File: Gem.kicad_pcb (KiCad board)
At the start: 2 copper layers, 56 x 54 mm, 40 parts, among them IC1 AD8226, IC2 AD8538, M1 ALLSENSORS-A6AAF-CUTLEADS, M2 DIAVOLINO, M6 ADAFRUIT-GPS-MOD, U1 ADS1115, U2 TCR2EF, U3 Micro-SD

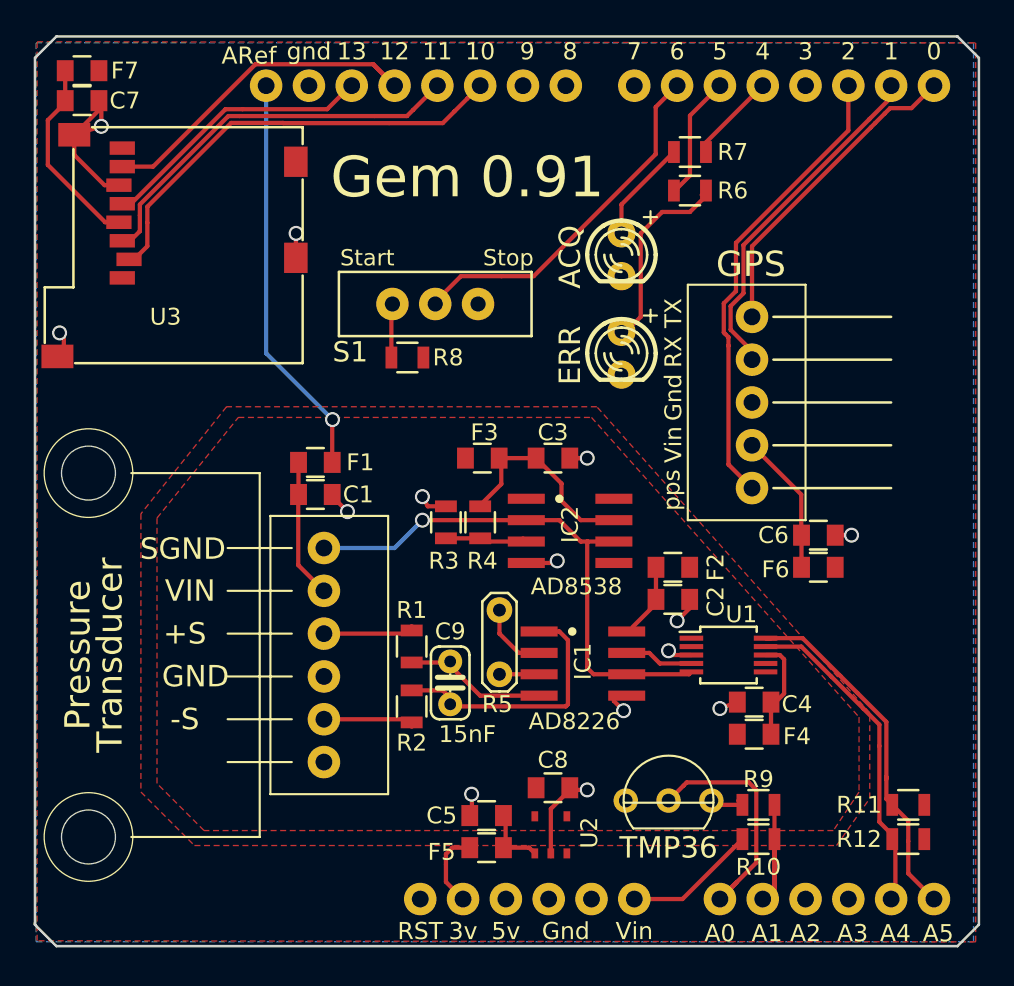
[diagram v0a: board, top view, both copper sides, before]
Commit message: v0.92, version of SRL paper
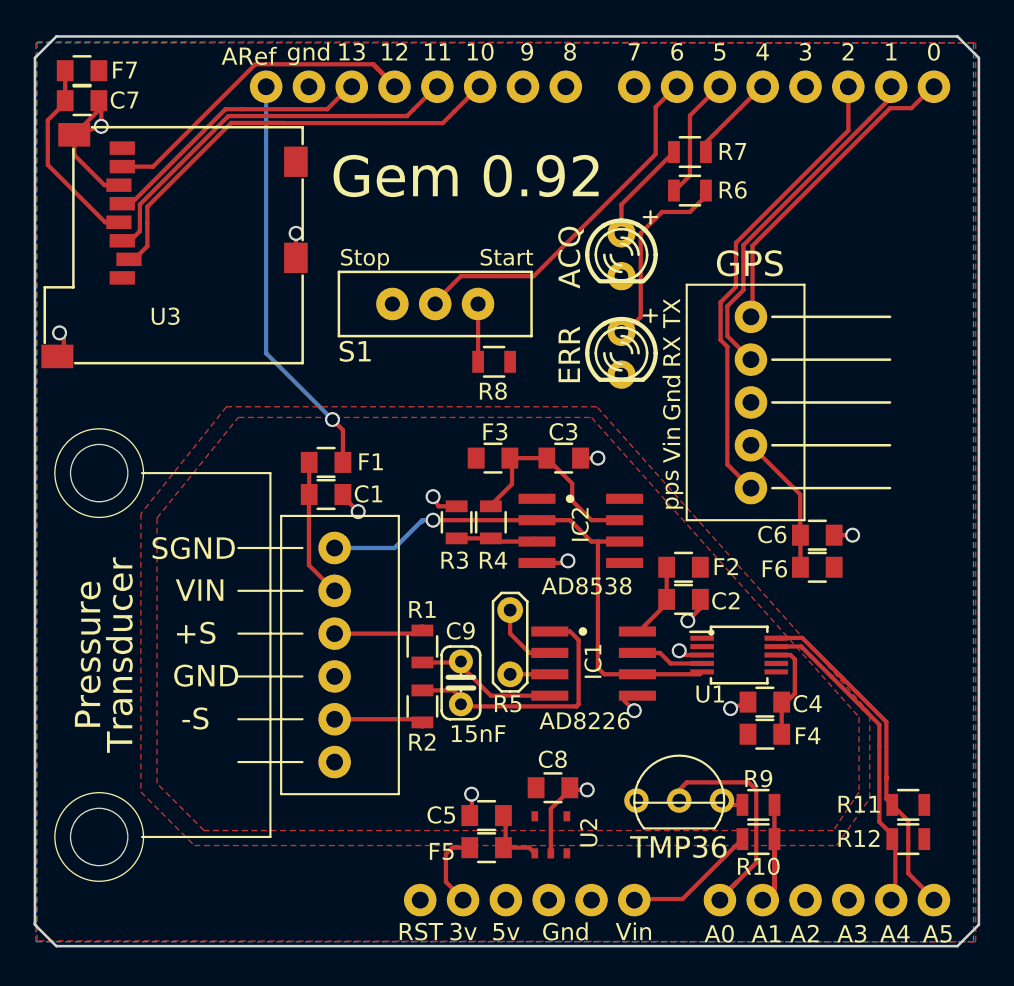
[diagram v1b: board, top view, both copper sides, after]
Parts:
- M2: value DIAVOLINO -> Board
- M6: value ADAFRUIT-GPS-MOD -> ADAFRUIT-GPS
- moved R8 5.15 mm to (29.8, 19.3)
- moved TMP36 0.64 mm to (40.8, 44.1)
- moved C1 0.64 mm to (19.8, 27.2)
- moved F1 0.64 mm to (19.8, 25.3)
- moved F3 0.64 mm to (29.7, 25.0)
- moved R1 0.64 mm to (25.5, 36.2)
- moved R2 0.64 mm to (25.5, 39.8)
- moved R3 0.64 mm to (27.6, 28.8)
- moved R4 0.64 mm to (29.6, 28.8)
- moved R5 0.64 mm to (30.7, 34.0)
- moved M1 0.63 mm to (6.35, 36.7)
- moved C2 0.63 mm to (41.0, 33.4)
- moved C3 0.63 mm to (33.9, 25.0)
- moved C4 0.63 mm to (45.8, 39.5)
- moved C9 0.63 mm to (27.8, 38.4)
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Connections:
- M2 pad 5V: Net-(M2-Pad5V) -> (no net)
- M2 pad A2: Net-(M2-PadA2) -> (no net)
- M2 pad A3: Net-(M2-PadA3) -> (no net)
- M2 pad D3: Net-(M2-PadD3) -> (no net)
- M2 pad D7: Net-(M2-PadD7) -> (no net)
- M2 pad D8: Net-(M2-PadD8) -> (no net)
- M2 pad D9: Net-(M2-PadD9) -> (no net)
- M2 pad RESE: Net-(M2-PadRESE) -> (no net)
- U1 pad 1: Net-(U1-Pad1) -> (no net)
- U1 pad 2: Net-(U1-Pad2) -> (no net)
- U1 pad 6: Net-(U1-Pad6) -> (no net)
- U1 pad 7: Net-(U1-Pad7) -> (no net)
- U2 pad 4: Net-(U2-Pad4) -> (no net)
- U3 pad 1: Net-(U3-Pad1) -> (no net)
- U3 pad 8: Net-(U3-Pad8) -> (no net)
- U3 pad 9: Net-(U3-Pad9) -> (no net)
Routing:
- net VAA: track 23.4 -> 24.3 mm
- net +1V5: track 32.8 -> 33.6 mm
- net /N$15: track 20.3 -> 20.9 mm
- net /N$20: track 19.5 -> 18.9 mm
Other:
- board text added: "Gem 0.92"
- board text removed: "Gem 0.91"

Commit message: v0.92, libraries fixed
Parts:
- C9: footprint Gem-modular:C025-024X044 -> Gem:C025-024X044
- IC1, IC2: footprint Gem-modular:SO8 -> Gem:SO8
- M1: footprint Gem-modular:ALLSENSORS-A6AAF-CUTLEADS -> Gem:ALLSENSORS-A6AAF-CUTLEADS
- M2: footprint Gem-modular:ARDUINO-NOHOLE-DIM_ON_BDOCU_ONLY -> Gem:ARDUINO-NOHOLE-DIM_ON_BDOCU_ONLY
- M6: footprint Gem-modular:ADAFRUIT-ULTIMATE-GPS-MOD -> Gem:ADAFRUIT-ULTIMATE-GPS-MOD
- R5: footprint Gem-modular:R-TH-VERT -> Gem:R-TH-VERT
- S1: footprint Gem-modular:EG1218 -> Gem:EG1218
- TMP36: footprint Gem-modular:TO92-EBC-OVAL -> Gem:TO92-EBC-OVAL
- U2: footprint Gem-modular:SC-74A -> Gem:SC-74A
- U3: footprint Gem-modular:Micro-SD -> Gem:Micro-SD
- blue1, red1: footprint Gem-modular:LED3MM -> Gem:LED3MM
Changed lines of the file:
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@@
     (add_net VAA)
   )
-  (module Gem-modular:ALLSENSORS-A6AAF-CUTLEADS (layer Top)
+  (module Gem:ALLSENSORS-A6AAF-CUTLEADS (layer Top)
     (at 6.35 36.703 270)
     (attr virtual)
@@
     (pad "" np_thru_hole circle (at 10.795 0 270) (size 3.4 3.4) (drill 3.4) (layers *.Cu *.Mask))
   )
-  (module Gem-modular:ARDUINO-NOHOLE-DIM_ON_BDOCU_ONLY locked (layer Top)
+  (module Gem:ARDUINO-NOHOLE-DIM_ON_BDOCU_ONLY locked (layer Top)
     (at 57.15 1.7145)
     (attr virtual)
@@
       (net 33 +BATT))
   )
-  (module Gem-modular:EG1218 (layer Top)
+  (module Gem:EG1218 (layer Top)
     (at 26.289 15.875 180)
     (fp_text reference S1 (at 5.7785 -3.556 360) (layer F.SilkS)
@@
       (net 31 GND))
   )
-  (module Gem-modular:ADAFRUIT-ULTIMATE-GPS-MOD (layer Top)
+  (module Gem:ADAFRUIT-ULTIMATE-GPS-MOD (layer Top)
     (at 58.3565 21.717)
     (attr virtual)
@@
       (net 20 /N$28))
   )
-  (module Gem-modular:SO8 (layer Top)
+  (module Gem:SO8 (layer Top)
     (at 35.687 37.211 270)
     (descr "8-LEAD SMALL OUTLINE IC (SO-8)")
@@
       (net 23 /N$31))
   )
-  (module Gem-modular:SO8 (layer Top)
+  (module Gem:SO8 (layer Top)
     (at 34.925 29.337 270)
     (descr "8-LEAD SMALL OUTLINE IC (SO-8)")
@@
     )
   )
-  (module Gem-modular:SC-74A (layer Top)
+  (module Gem:SC-74A (layer Top)
     (at 33.147 47.371)
     (fp_text reference U2 (at 2.286 -0.127 90) (layer F.SilkS)
@@
       (net 34 "Net-(C5-Pad2)"))
   )
-  (module Gem-modular:LED3MM (layer Top)
+  (module Gem:LED3MM (layer Top)
     (at 37.338 18.796 270)
     (descr LED)
@@
       (net 31 GND))
   )
-  (module Gem-modular:LED3MM (layer Top)
+  (module Gem:LED3MM (layer Top)
     (at 37.338 12.954 270)
     (descr LED)
@@
       (net 31 GND))
   )
-  (module Gem-modular:Micro-SD (layer Top)
+  (module Gem:Micro-SD (layer Top)
     (at 2.921 19.685 90)
     (fp_text reference U3 (at 3.048 7.366 180) (layer F.SilkS)
@@
       (net 31 GND))
   )
-  (module Gem-modular:TO92-EBC-OVAL (layer Top)
+  (module Gem:TO92-EBC-OVAL (layer Top)
     (at 40.767 44.069)
     (descr TO-92)
@@
     )
   )
-  (module Gem-modular:C025-024X044 (layer Top)
+  (module Gem:C025-024X044 (layer Top)
     (at 27.813 38.354 90)
     (descr CAPACITOR)
@@
     )
   )
-  (module Gem-modular:R-TH-VERT (layer Top)
+  (module Gem:R-TH-VERT (layer Top)
     (at 30.734 34.036 90)
     (fp_text reference R5 (at -5.588 -0.127 180) (layer F.SilkS)
